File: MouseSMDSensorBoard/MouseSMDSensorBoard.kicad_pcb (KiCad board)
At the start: 2 copper layers, 18 x 35 mm, 18 parts, among them J1 Conn_01x05

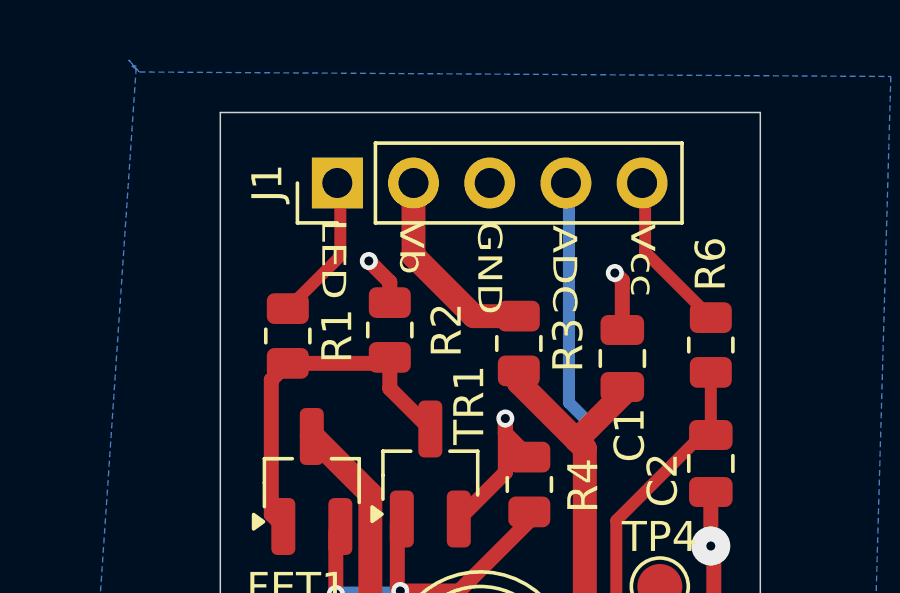
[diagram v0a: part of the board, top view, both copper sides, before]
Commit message: Sort of ready for JLCPCB
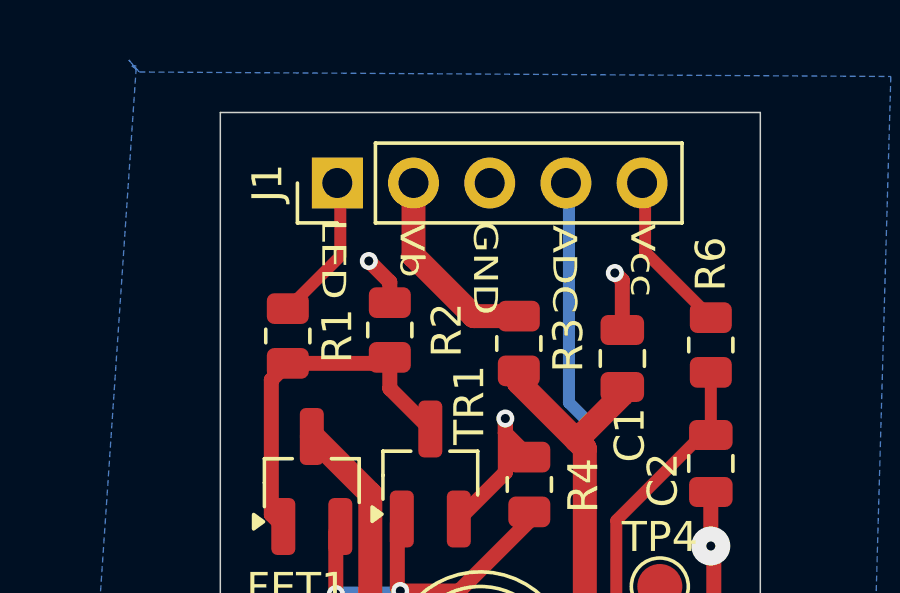
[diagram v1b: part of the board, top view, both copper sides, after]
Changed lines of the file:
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@@
 	)
 	(gr_text "GND"
-		(at 142 77.05 90)
+		(at 141.87 77.06 90)
 		(layer "B.SilkS")
 		(effects
@@
 	)
 	(gr_text "GND"
-		(at 141 77.05 -90)
+		(at 140.86 77.06 -90)
 		(layer "F.SilkS")
 		(effects
@@
 	)
 	(gr_text "Vb\n"
-		(at 138.4 77.05 270)
+		(at 138.41 77.15 270)
 		(layer "F.SilkS")
 		(effects
